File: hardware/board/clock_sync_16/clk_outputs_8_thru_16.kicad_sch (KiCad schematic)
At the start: 40 parts, among them J2 AudioJack3, U5 ISO6521FREUR

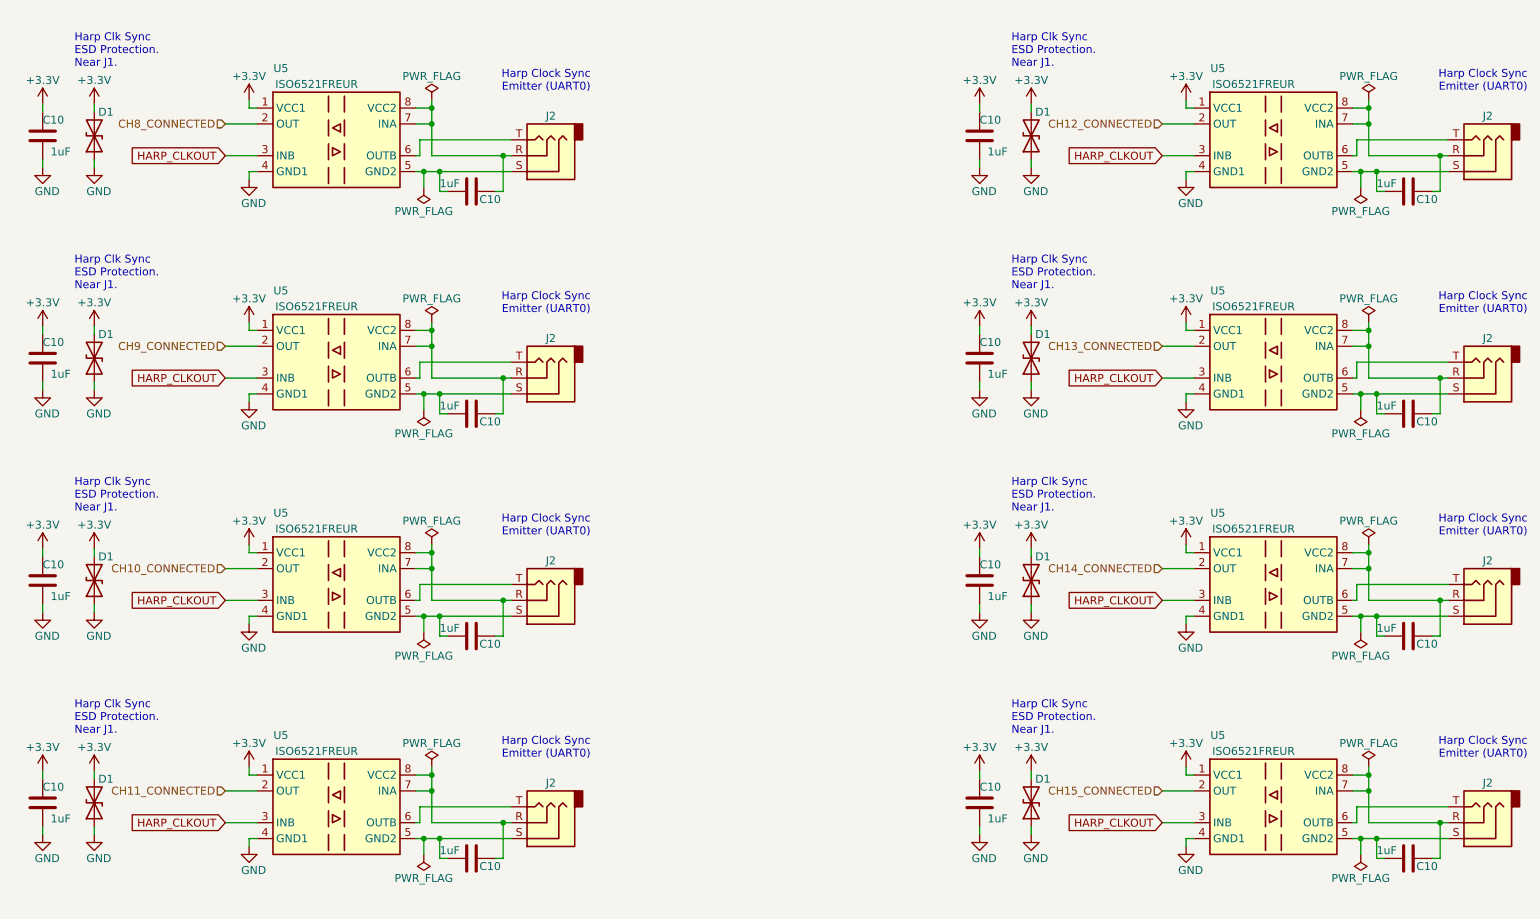
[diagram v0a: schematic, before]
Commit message: route pcb v0.1
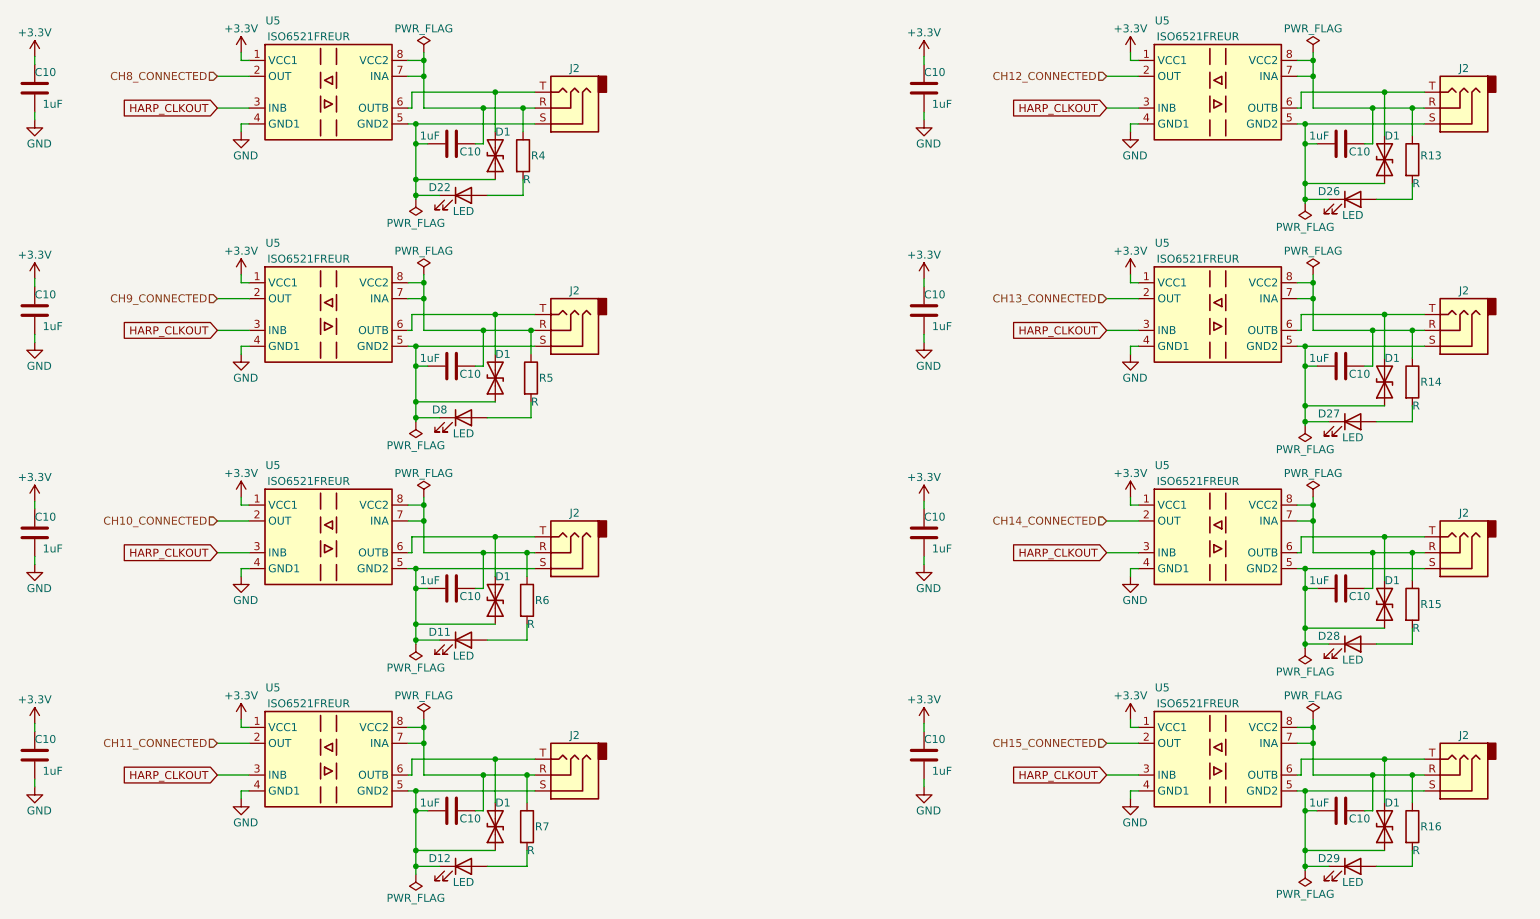
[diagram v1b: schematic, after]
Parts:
- removed C10 (x16): 1uF, Capacitor_SMD:C_0402_1005Metric, symbol Device:C
- removed D1 (x8): D_TVS, Diode_SMD:D_0402_1005Metric, symbol Device:D_TVS
- removed J2 (x8): AudioJack3, Connector_Audio:Jack_3.5mm_CUI_SJ-3523-SMT_Horizontal, symbol Connector:AudioJack3
- removed U5 (x8): ISO6521FREUR, kicad_component_library:DFN-8_3x2mm_P0.5mm, symbol kicad_component_library:ISO6521FREUR
- added C10 (x16): 1uF, Capacitor_SMD:C_0402_1005Metric, symbol Device:C
- added D1 (x8): D_TVS, Diode_SMD:D_0402_1005Metric, symbol Device:D_TVS
- added D11, D12, D22, D26, D27, D28, D29, D8: LED, LED_SMD:LED_0603_1608Metric_Pad1.05x0.95mm_HandSolder, symbol Device:LED
- added J2 (x8): AudioJack3, kicad_component_library:Jack_3.5mm_Kycon_STX-3680-5NB_Vertical, symbol Connector:AudioJack3
- added R13, R14, R15, R16, R4, R5, R6, R7: R, Resistor_SMD:R_0402_1005Metric, symbol Device:R
- added U5 (x8): ISO6521FREUR, kicad_component_library:DFN-8_3x2mm_P0.5mm, symbol kicad_component_library:ISO6521FREUR
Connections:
- net +3.3V: now also C10.1, C10.1, C10.1, C10.1, C10.1, C10.1, C10.1, C10.1, U5.1 (VCC1), U5.1 (VCC1), U5.1 (VCC1), U5.1 (VCC1), U5.1 (VCC1), U5.1 (VCC1), U5.1 (VCC1), U5.1 (VCC1)
- net CH10_CONNECTED: now also U5.2 (OUT)
- net CH11_CONNECTED: now also U5.2 (OUT)
- net CH12_CONNECTED: now also U5.2 (OUT)
- net CH13_CONNECTED: now also U5.2 (OUT)
- net CH14_CONNECTED: now also U5.2 (OUT)
- net CH15_CONNECTED: now also U5.2 (OUT)
- net CH8_CONNECTED: now also U5.2 (OUT)
- net CH9_CONNECTED: now also U5.2 (OUT)
- net GND: now also C10.2, C10.2, C10.2, C10.2, C10.2, C10.2, C10.2, C10.2, U5.4 (GND1), U5.4 (GND1), U5.4 (GND1), U5.4 (GND1), U5.4 (GND1), U5.4 (GND1), U5.4 (GND1), U5.4 (GND1)
- net HARP_CLKOUT: now also U5.3 (INB), U5.3 (INB), U5.3 (INB), U5.3 (INB), U5.3 (INB), U5.3 (INB), U5.3 (INB), U5.3 (INB)
- new net: C10.2, D1.1 (A1), D28.1 (K), J2.S, U5.5 (GND2)
- new net: D1.2 (A2), J2.T, U5.6 (OUTB) (x8)
- new net: C10.1, J2.R, R15.1, U5.7 (INA), U5.8 (VCC2)
- new net: C10.2, D1.1 (A1), D29.1 (K), J2.S, U5.5 (GND2)
- new net: C10.2, D1.1 (A1), D26.1 (K), J2.S, U5.5 (GND2)
- new net: C10.1, J2.R, R4.1, U5.7 (INA), U5.8 (VCC2)
- new net: C10.2, D1.1 (A1), D22.1 (K), J2.S, U5.5 (GND2)
- new net: C10.2, D1.1 (A1), D11.1 (K), J2.S, U5.5 (GND2)
- new net: C10.2, D1.1 (A1), D8.1 (K), J2.S, U5.5 (GND2)
- new net: C10.1, J2.R, R14.1, U5.7 (INA), U5.8 (VCC2)
- new net: C10.2, D1.1 (A1), D27.1 (K), J2.S, U5.5 (GND2)
- new net: D27.2 (A), R14.2
- new net: C10.1, J2.R, R13.1, U5.7 (INA), U5.8 (VCC2)
- new net: D28.2 (A), R15.2
- new net: C10.1, J2.R, R6.1, U5.7 (INA), U5.8 (VCC2)
- new net: D11.2 (A), R6.2
- new net: D8.2 (A), R5.2
- new net: C10.1, J2.R, R5.1, U5.7 (INA), U5.8 (VCC2)
- new net: D29.2 (A), R16.2
- new net: C10.1, J2.R, R16.1, U5.7 (INA), U5.8 (VCC2)
- new net: C10.2, D1.1 (A1), D12.1 (K), J2.S, U5.5 (GND2)
- new net: D12.2 (A), R7.2
- new net: C10.1, J2.R, R7.1, U5.7 (INA), U5.8 (VCC2)
- new net: D26.2 (A), R13.2
- new net: D22.2 (A), R4.2
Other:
- note removed: "Harp Clk Sync ESD Protection. Near J1."
- note removed: "Harp Clock Sync Emitter (UART0)"
